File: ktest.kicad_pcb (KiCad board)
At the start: 4 copper layers, 100 x 100 mm, 46 parts, among them J1 Conn_01x03_Pin, U1 STM32WBA55HEFx

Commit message: change folder structure
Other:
- board text added: "IPC In case of divergences, dimensions from Gerber files take precedence Surface finish: Lead-free HASL, Copper thickness: minimum x um external layer, minimum x internal layer, per IPC xxx vias to be left untended / tented / filled and capped process must be RoHS compliant flammability rating shall meet as a minimum ul94v-0 tg170 or better tolerance xxx or as per ipc"

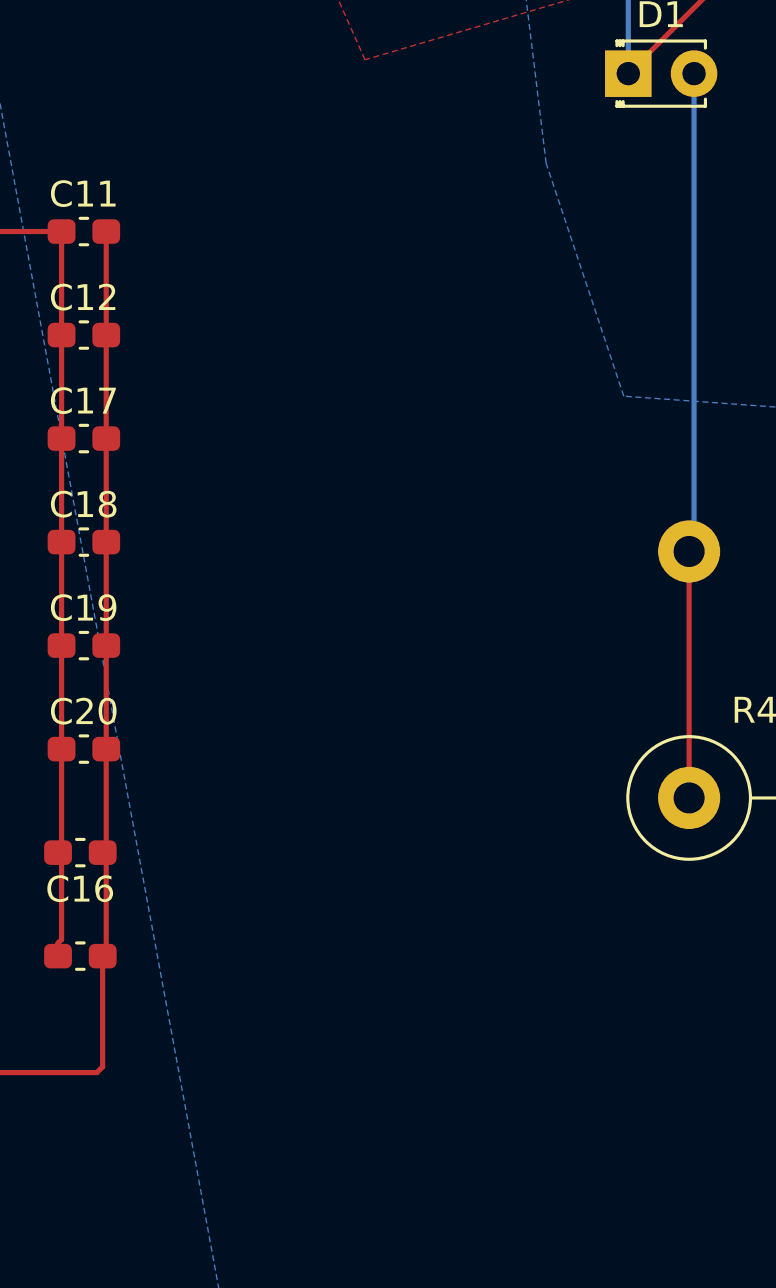
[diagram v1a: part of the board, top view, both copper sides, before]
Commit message: testing erc bypass
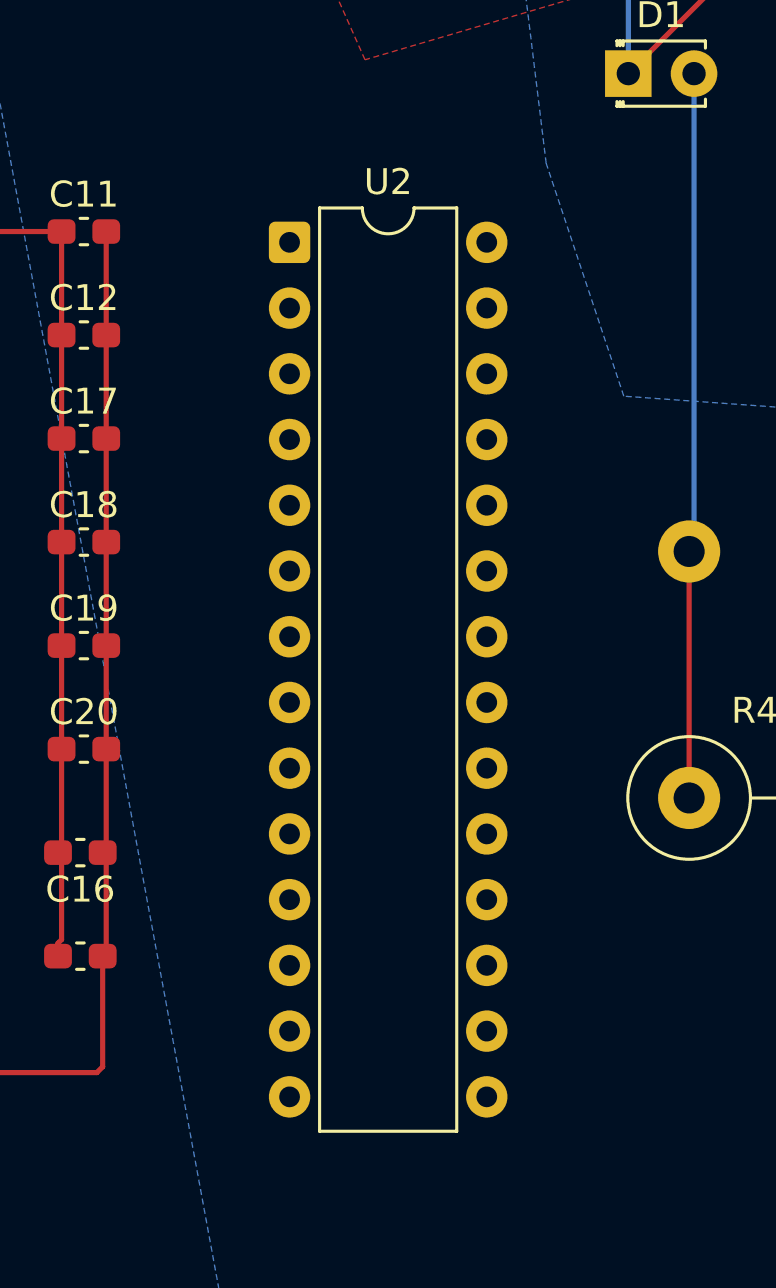
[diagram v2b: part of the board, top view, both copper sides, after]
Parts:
- added U2: ATmega8-16P, Package_DIP:DIP-28_W7.62mm, F.Cu at (100.1, 87.1)

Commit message: testing both erc drc overlay
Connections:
- U2 pad 14: unconnected-(U2-PB0-Pad14) -> Net-(U2-PB0)
- U2 pad 15: unconnected-(U2-PB1-Pad15) -> Net-(U2-PB0)
- U2 pad 16: unconnected-(U2-PB2-Pad16) -> Net-(U2-PB0)
- U2 pad 17: unconnected-(U2-PB3-Pad17) -> Net-(U2-PB0)
- U2 pad 18: unconnected-(U2-PB4-Pad18) -> Net-(U2-PB0)
- U2 pad 19: unconnected-(U2-PB5-Pad19) -> Net-(U2-PB0)
- U2 pad 2: unconnected-(U2-PD0-Pad2) -> Net-(U2-PB0)
- U2 pad 23: unconnected-(U2-PC0-Pad23) -> Net-(U2-PB0)
- U2 pad 24: unconnected-(U2-PC1-Pad24) -> Net-(U2-PB0)
- U2 pad 25: unconnected-(U2-PC2-Pad25) -> Net-(U2-PB0)
- U2 pad 26: unconnected-(U2-PC3-Pad26) -> Net-(U2-PB0)
- U2 pad 27: unconnected-(U2-PC4-Pad27) -> Net-(U2-PB0)
- U2 pad 28: unconnected-(U2-PC5-Pad28) -> Net-(U2-PB0)
- U2 pad 3: unconnected-(U2-PD1-Pad3) -> Net-(U2-PB0)
- U2 pad 4: unconnected-(U2-PD2-Pad4) -> Net-(U2-PB0)
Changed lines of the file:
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@@
 			(layers "*.Cu" "*.Mask")
 			(remove_unused_layers no)
-			(net "unconnected-(U2-PD0-Pad2)")
+			(net "Net-(U2-PB0)")
 			(pinfunction "PD0_2")
 			(pintype "bidirectional")
@@
 			(layers "*.Cu" "*.Mask")
 			(remove_unused_layers no)
-			(net "unconnected-(U2-PD1-Pad3)")
+			(net "Net-(U2-PB0)")
 			(pinfunction "PD1_3")
 			(pintype "bidirectional")
@@
 			(layers "*.Cu" "*.Mask")
 			(remove_unused_layers no)
-			(net "unconnected-(U2-PD2-Pad4)")
+			(net "Net-(U2-PB0)")
 			(pinfunction "PD2_4")
 			(pintype "bidirectional")
@@
 			(layers "*.Cu" "*.Mask")
 			(remove_unused_layers no)
-			(net "unconnected-(U2-PB0-Pad14)")
+			(net "Net-(U2-PB0)")
 			(pinfunction "PB0_14")
 			(pintype "bidirectional")
@@
 			(layers "*.Cu" "*.Mask")
 			(remove_unused_layers no)
-			(net "unconnected-(U2-PB1-Pad15)")
+			(net "Net-(U2-PB0)")
 			(pinfunction "PB1_15")
 			(pintype "bidirectional")
@@
 			(layers "*.Cu" "*.Mask")
 			(remove_unused_layers no)
-			(net "unconnected-(U2-PB2-Pad16)")
+			(net "Net-(U2-PB0)")
 			(pinfunction "PB2_16")
 			(pintype "bidirectional")
@@
 			(layers "*.Cu" "*.Mask")
 			(remove_unused_layers no)
-			(net "unconnected-(U2-PB3-Pad17)")
+			(net "Net-(U2-PB0)")
 			(pinfunction "PB3_17")
 			(pintype "bidirectional")
@@
 			(layers "*.Cu" "*.Mask")
 			(remove_unused_layers no)
-			(net "unconnected-(U2-PB4-Pad18)")
+			(net "Net-(U2-PB0)")
 			(pinfunction "PB4_18")
 			(pintype "bidirectional")
@@
 			(layers "*.Cu" "*.Mask")
 			(remove_unused_layers no)
-			(net "unconnected-(U2-PB5-Pad19)")
+			(net "Net-(U2-PB0)")
 			(pinfunction "PB5_19")
 			(pintype "bidirectional")
@@
 			(layers "*.Cu" "*.Mask")
 			(remove_unused_layers no)
-			(net "unconnected-(U2-PC0-Pad23)")
+			(net "Net-(U2-PB0)")
 			(pinfunction "PC0_23")
 			(pintype "bidirectional")
@@
 			(layers "*.Cu" "*.Mask")
 			(remove_unused_layers no)
-			(net "unconnected-(U2-PC1-Pad24)")
+			(net "Net-(U2-PB0)")
 			(pinfunction "PC1_24")
 			(pintype "bidirectional")
@@
 			(layers "*.Cu" "*.Mask")
 			(remove_unused_layers no)
-			(net "unconnected-(U2-PC2-Pad25)")
+			(net "Net-(U2-PB0)")
 			(pinfunction "PC2_25")
 			(pintype "bidirectional")
@@
 			(layers "*.Cu" "*.Mask")
 			(remove_unused_layers no)
-			(net "unconnected-(U2-PC3-Pad26)")
+			(net "Net-(U2-PB0)")
 			(pinfunction "PC3_26")
 			(pintype "bidirectional")
@@
 			(layers "*.Cu" "*.Mask")
 			(remove_unused_layers no)
-			(net "unconnected-(U2-PC4-Pad27)")
+			(net "Net-(U2-PB0)")
 			(pinfunction "PC4_27")
 			(pintype "bidirectional")
@@
 			(layers "*.Cu" "*.Mask")
 			(remove_unused_layers no)
-			(net "unconnected-(U2-PC5-Pad28)")
+			(net "Net-(U2-PB0)")
 			(pinfunction "PC5_28")
 			(pintype "bidirectional")

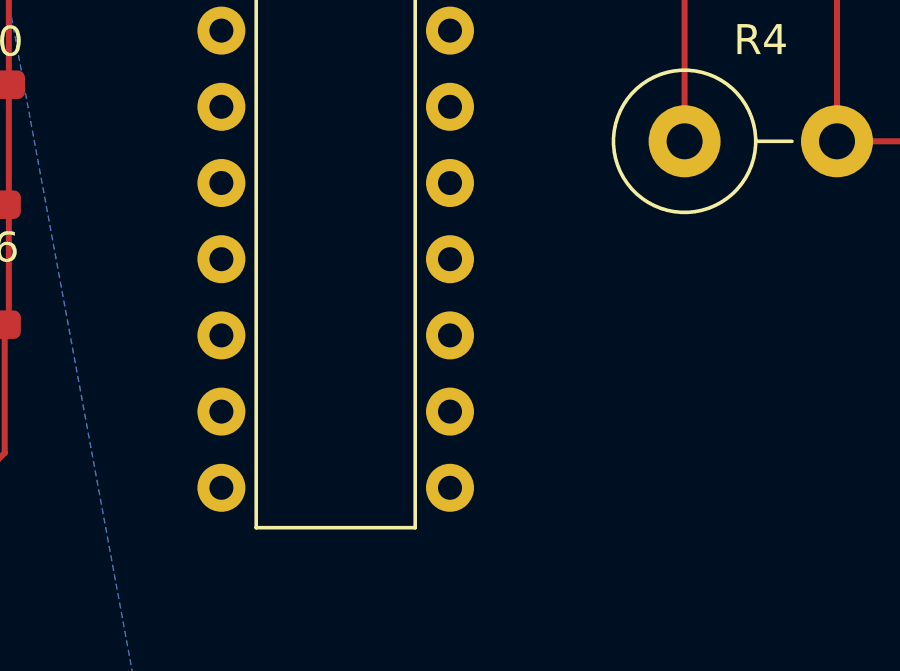
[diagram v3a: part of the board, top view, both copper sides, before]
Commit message: testing drc bypass only
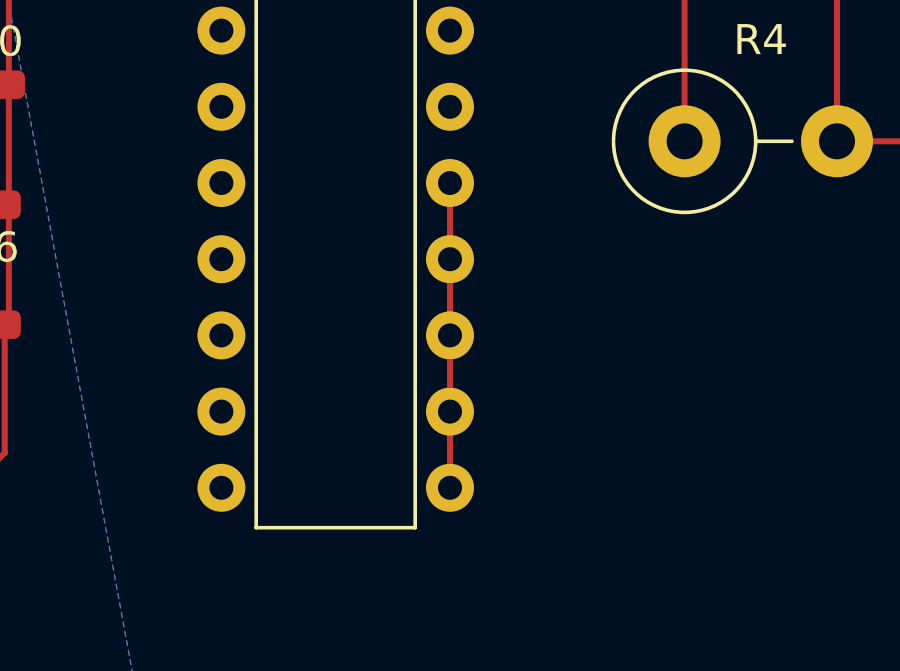
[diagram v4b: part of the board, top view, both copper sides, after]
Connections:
- U2 pad 14: Net-(U2-PB0) -> unconnected-(U2-PB0-Pad14)
- U2 pad 15: Net-(U2-PB0) -> unconnected-(U2-PB1-Pad15)
- U2 pad 16: Net-(U2-PB0) -> unconnected-(U2-PB2-Pad16)
- U2 pad 17: Net-(U2-PB0) -> unconnected-(U2-PB3-Pad17)
- U2 pad 18: Net-(U2-PB0) -> unconnected-(U2-PB4-Pad18)
- U2 pad 19: Net-(U2-PB0) -> unconnected-(U2-PB5-Pad19)
- U2 pad 2: Net-(U2-PB0) -> unconnected-(U2-PD0-Pad2)
- U2 pad 23: Net-(U2-PB0) -> unconnected-(U2-PC0-Pad23)
- U2 pad 24: Net-(U2-PB0) -> unconnected-(U2-PC1-Pad24)
- U2 pad 25: Net-(U2-PB0) -> unconnected-(U2-PC2-Pad25)
- U2 pad 26: Net-(U2-PB0) -> unconnected-(U2-PC3-Pad26)
- U2 pad 27: Net-(U2-PB0) -> unconnected-(U2-PC4-Pad27)
- U2 pad 28: Net-(U2-PB0) -> unconnected-(U2-PC5-Pad28)
- U2 pad 3: Net-(U2-PB0) -> unconnected-(U2-PD1-Pad3)
- U2 pad 4: Net-(U2-PB0) -> unconnected-(U2-PD2-Pad4)
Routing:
- net (no net): track 0.00 -> 10.2 mm
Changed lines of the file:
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@@
 			(net "unconnected-(U2-PC6{slash}~{RESET}-Pad1)")
 			(pinfunction "PC6/~{RESET}_1")
-			(pintype "bidirectional")
+			(pintype "bidirectional+no_connect")
 		)
 		(pad "2" thru_hole circle
@@
 			(layers "*.Cu" "*.Mask")
 			(remove_unused_layers no)
-			(net "Net-(U2-PB0)")
+			(net "unconnected-(U2-PD0-Pad2)")
 			(pinfunction "PD0_2")
-			(pintype "bidirectional")
+			(pintype "bidirectional+no_connect")
 		)
 		(pad "3" thru_hole circle
@@
 			(layers "*.Cu" "*.Mask")
 			(remove_unused_layers no)
-			(net "Net-(U2-PB0)")
+			(net "unconnected-(U2-PD1-Pad3)")
 			(pinfunction "PD1_3")
-			(pintype "bidirectional")
+			(pintype "bidirectional+no_connect")
 		)
 		(pad "4" thru_hole circle
@@
 			(layers "*.Cu" "*.Mask")
 			(remove_unused_layers no)
-			(net "Net-(U2-PB0)")
+			(net "unconnected-(U2-PD2-Pad4)")
 			(pinfunction "PD2_4")
-			(pintype "bidirectional")
+			(pintype "bidirectional+no_connect")
 		)
 		(pad "5" thru_hole circle
@@
 			(net "unconnected-(U2-PD3-Pad5)")
 			(pinfunction "PD3_5")
-			(pintype "bidirectional")
+			(pintype "bidirectional+no_connect")
 		)
 		(pad "6" thru_hole circle
@@
 			(net "unconnected-(U2-PD4-Pad6)")
 			(pinfunction "PD4_6")
-			(pintype "bidirectional")
+			(pintype "bidirectional+no_connect")
 		)
 		(pad "7" thru_hole circle
@@
 			(net "unconnected-(U2-VCC-Pad7)")
 			(pinfunction "VCC_7")
-			(pintype "power_in")
+			(pintype "power_in+no_connect")
 		)
 		(pad "8" thru_hole circle
@@
 			(net "unconnected-(U2-GND-Pad8)")
 			(pinfunction "GND_8")
-			(pintype "power_in")
+			(pintype "power_in+no_connect")
 		)
 		(pad "9" thru_hole circle
@@
 			(net "unconnected-(U2-PB6{slash}XTAL1-Pad9)")
 			(pinfunction "PB6/XTAL1_9")
-			(pintype "bidirectional")
+			(pintype "bidirectional+no_connect")
 		)
 		(pad "10" thru_hole circle
@@
 			(net "unconnected-(U2-PB7{slash}XTAL2-Pad10)")
 			(pinfunction "PB7/XTAL2_10")
-			(pintype "bidirectional")
+			(pintype "bidirectional+no_connect")
 		)
 		(pad "11" thru_hole circle
@@
 			(net "unconnected-(U2-PD5-Pad11)")
 			(pinfunction "PD5_11")
-			(pintype "bidirectional")
+			(pintype "bidirectional+no_connect")
 		)
 		(pad "12" thru_hole circle
@@
 			(net "unconnected-(U2-PD6-Pad12)")
 			(pinfunction "PD6_12")
-			(pintype "bidirectional")
+			(pintype "bidirectional+no_connect")
 		)
 		(pad "13" thru_hole circle
@@
 			(net "unconnected-(U2-PD7-Pad13)")
 			(pinfunction "PD7_13")
-			(pintype "bidirectional")
+			(pintype "bidirectional+no_connect")
 		)
 		(pad "14" thru_hole circle
@@
 			(layers "*.Cu" "*.Mask")
 			(remove_unused_layers no)
-			(net "Net-(U2-PB0)")
+			(net "unconnected-(U2-PB0-Pad14)")
 			(pinfunction "PB0_14")
-			(pintype "bidirectional")
+			(pintype "bidirectional+no_connect")
 		)
 		(pad "15" thru_hole circle
@@
 			(layers "*.Cu" "*.Mask")
 			(remove_unused_layers no)
-			(net "Net-(U2-PB0)")
+			(net "unconnected-(U2-PB1-Pad15)")
 			(pinfunction "PB1_15")
-			(pintype "bidirectional")
+			(pintype "bidirectional+no_connect")
 		)
 		(pad "16" thru_hole circle
@@
 			(layers "*.Cu" "*.Mask")
 			(remove_unused_layers no)
-			(net "Net-(U2-PB0)")
+			(net "unconnected-(U2-PB2-Pad16)")
 			(pinfunction "PB2_16")
-			(pintype "bidirectional")
+			(pintype "bidirectional+no_connect")
 		)
 		(pad "17" thru_hole circle
@@
 			(layers "*.Cu" "*.Mask")
 			(remove_unused_layers no)
-			(net "Net-(U2-PB0)")
+			(net "unconnected-(U2-PB3-Pad17)")
 			(pinfunction "PB3_17")
-			(pintype "bidirectional")
+			(pintype "bidirectional+no_connect")
 		)
 		(pad "18" thru_hole circle
@@
 			(layers "*.Cu" "*.Mask")
 			(remove_unused_layers no)
-			(net "Net-(U2-PB0)")
+			(net "unconnected-(U2-PB4-Pad18)")
 			(pinfunction "PB4_18")
-			(pintype "bidirectional")
+			(pintype "bidirectional+no_connect")
 		)
 		(pad "19" thru_hole circle
@@
 			(layers "*.Cu" "*.Mask")
 			(remove_unused_layers no)
-			(net "Net-(U2-PB0)")
+			(net "unconnected-(U2-PB5-Pad19)")
 			(pinfunction "PB5_19")
-			(pintype "bidirectional")
+			(pintype "bidirectional+no_connect")
 		)
 		(pad "20" thru_hole circle
@@
 			(net "unconnected-(U2-AVCC-Pad20)")
 			(pinfunction "AVCC_20")
-			(pintype "power_in")
+			(pintype "power_in+no_connect")
 		)
 		(pad "21" thru_hole circle
@@
 			(net "unconnected-(U2-AREF-Pad21)")
 			(pinfunction "AREF_21")
-			(pintype "passive")
+			(pintype "passive+no_connect")
 		)
 		(pad "22" thru_hole circle
@@
 			(net "unconnected-(U2-AGND-Pad22)")
 			(pinfunction "AGND_22")
-			(pintype "power_in")
+			(pintype "power_in+no_connect")
 		)
 		(pad "23" thru_hole circle
@@
 			(layers "*.Cu" "*.Mask")
 			(remove_unused_layers no)
-			(net "Net-(U2-PB0)")
+			(net "unconnected-(U2-PC0-Pad23)")
 			(pinfunction "PC0_23")
-			(pintype "bidirectional")
+			(pintype "bidirectional+no_connect")
 		)
 		(pad "24" thru_hole circle
@@
 			(layers "*.Cu" "*.Mask")
 			(remove_unused_layers no)
-			(net "Net-(U2-PB0)")
+			(net "unconnected-(U2-PC1-Pad24)")
 			(pinfunction "PC1_24")
-			(pintype "bidirectional")
+			(pintype "bidirectional+no_connect")
 		)
 		(pad "25" thru_hole circle
@@
 			(layers "*.Cu" "*.Mask")
 			(remove_unused_layers no)
-			(net "Net-(U2-PB0)")
+			(net "unconnected-(U2-PC2-Pad25)")
 			(pinfunction "PC2_25")
-			(pintype "bidirectional")
+			(pintype "bidirectional+no_connect")
 		)
 		(pad "26" thru_hole circle
@@
 			(layers "*.Cu" "*.Mask")
 			(remove_unused_layers no)
-			(net "Net-(U2-PB0)")
+			(net "unconnected-(U2-PC3-Pad26)")
 			(pinfunction "PC3_26")
-			(pintype "bidirectional")
+			(pintype "bidirectional+no_connect")
 		)
 		(pad "27" thru_hole circle
@@
 			(layers "*.Cu" "*.Mask")
 			(remove_unused_layers no)
-			(net "Net-(U2-PB0)")
+			(net "unconnected-(U2-PC4-Pad27)")
 			(pinfunction "PC4_27")
-			(pintype "bidirectional")
+			(pintype "bidirectional+no_connect")
 		)
 		(pad "28" thru_hole circle
@@
 			(layers "*.Cu" "*.Mask")
 			(remove_unused_layers no)
-			(net "Net-(U2-PB0)")
+			(net "unconnected-(U2-PC5-Pad28)")
 			(pinfunction "PC5_28")
-			(pintype "bidirectional")
+			(pintype "bidirectional+no_connect")
 		)
 		(embedded_fonts no)
@@
 	)
 	(segment
+		(start 107.705 120.075)
+		(end 107.705 109.915)
+		(width 0.2)
+		(layer "F.Cu")
+		(net "")
+	)
+	(segment

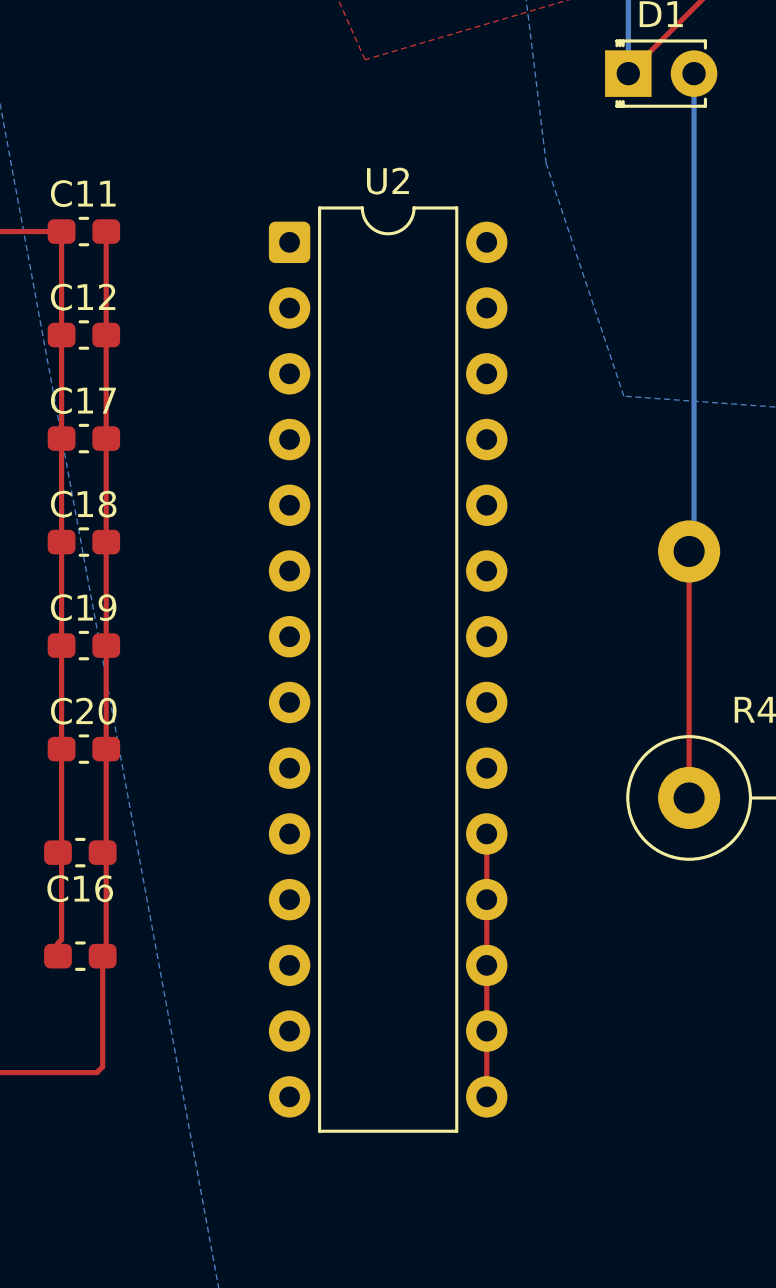
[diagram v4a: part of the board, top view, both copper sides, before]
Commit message: merging scripts
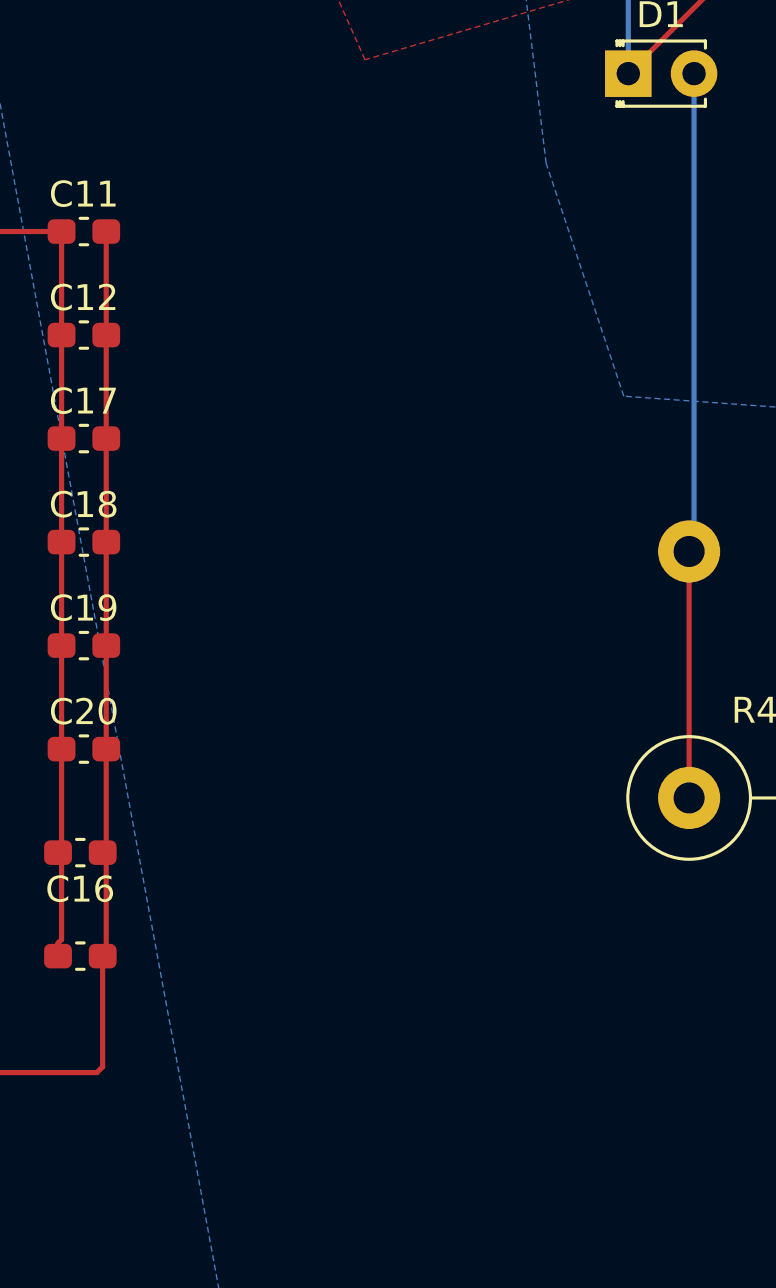
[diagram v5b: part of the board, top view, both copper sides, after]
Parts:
- removed U2: ATmega8-16P, Package_DIP:DIP-28_W7.62mm
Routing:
- net (no net): track 10.2 -> 0.00 mm
